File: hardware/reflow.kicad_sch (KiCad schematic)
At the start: 45 parts, among them K1 OZ-SS-112L1, K2 OZ-SS-112L1, K3 SDT-SS-112DM, K4 0J-SS-112LWHF, Q1 RE1C002UNTCL, Q2 RE1C002UNTCL, Q3 RE1C002UNTCL, Q4 RE1C002UNTCL, U1 ESP-12E, U2 AD8495

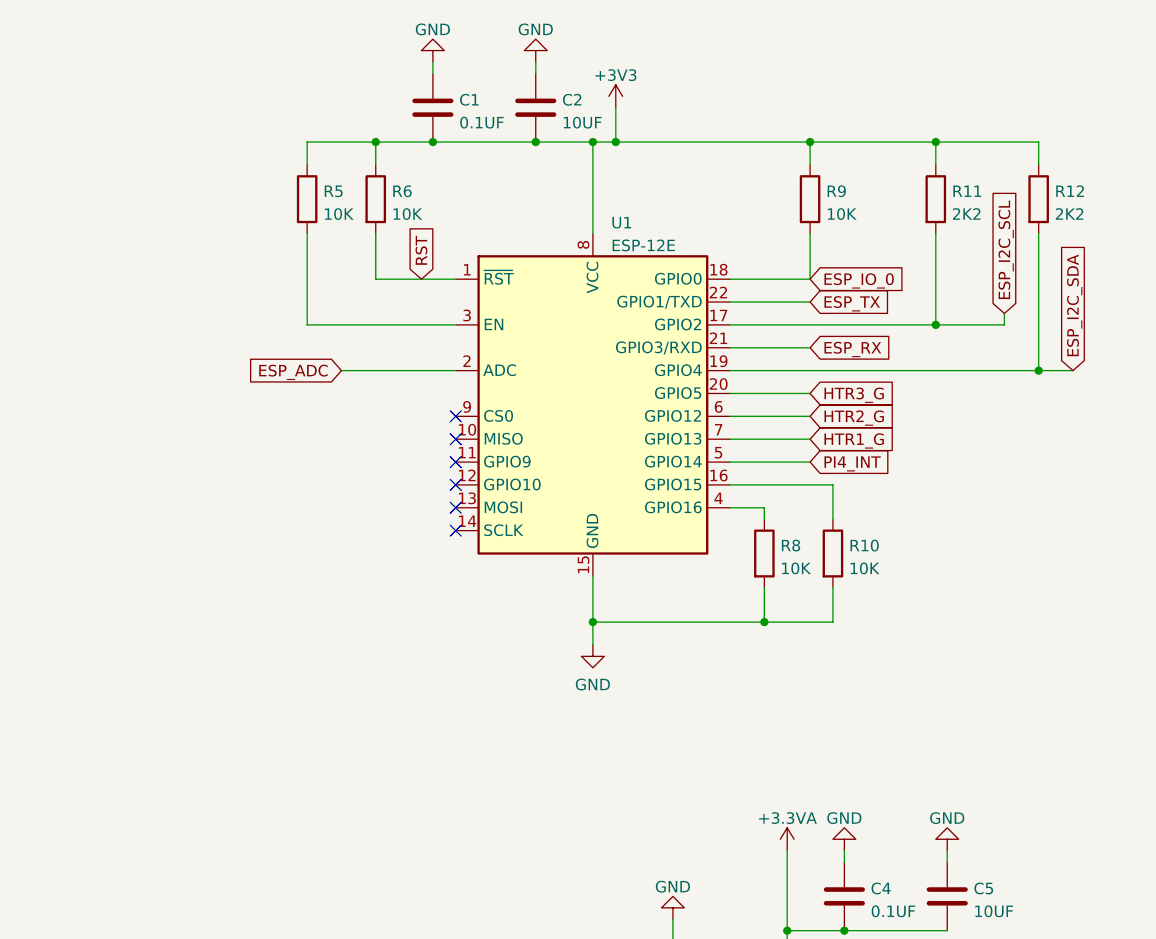
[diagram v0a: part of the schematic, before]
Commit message: updated kicad files
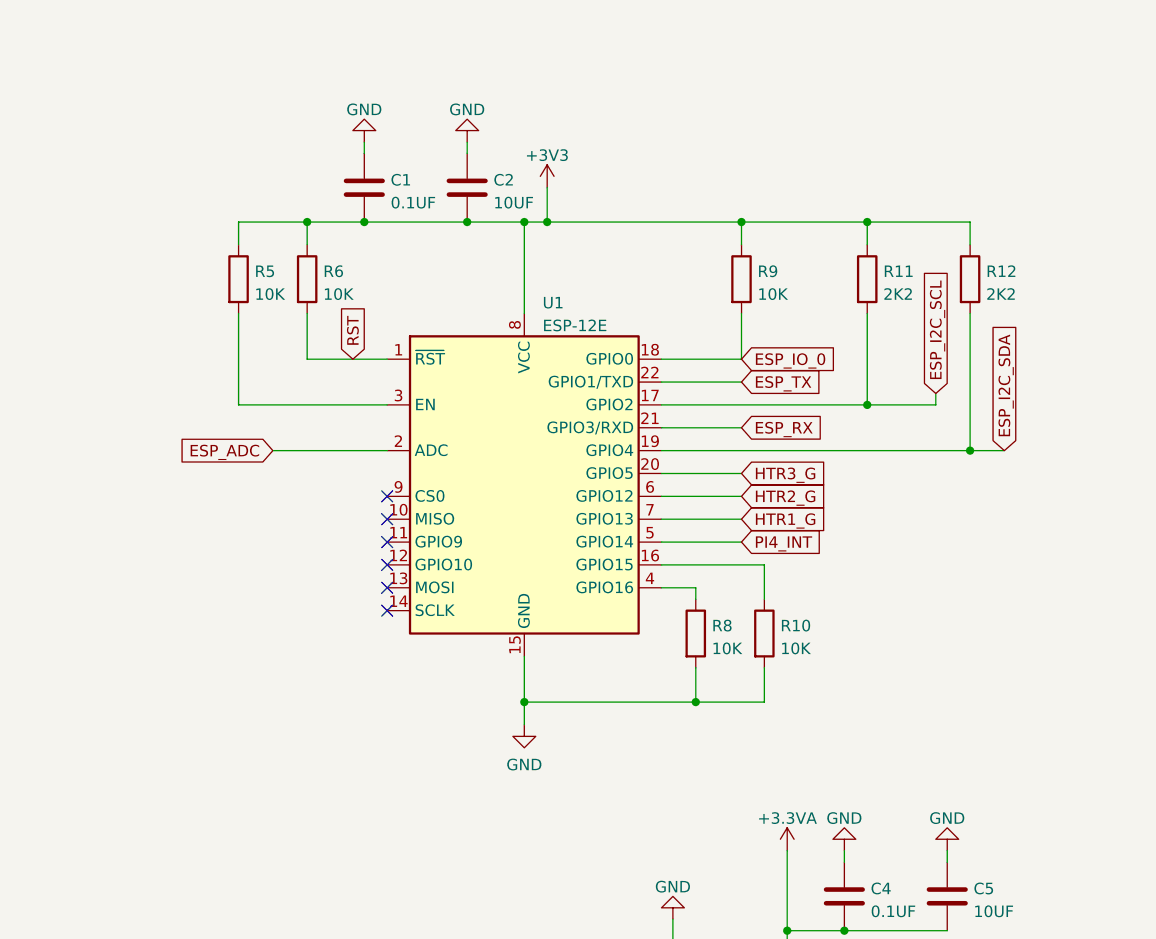
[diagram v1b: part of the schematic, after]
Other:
- moved on the sheet: C1, C2, R10, R11, R12, R5, R6, R8, R9, U1
